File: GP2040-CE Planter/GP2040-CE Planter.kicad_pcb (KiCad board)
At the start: 4 copper layers, 50 x 50 mm, 57 parts, among them J1 USB_B, J2 USB_A, J3 USB_A, J4 USB_A, J5 USB_A, J6 USB_A, J7 Conn_01x02, U1 TUSB4041IPAPR, U3 TPS2561ADRCR, U4 TPS2561ADRCR, U5 PTMUXHS221NKGR

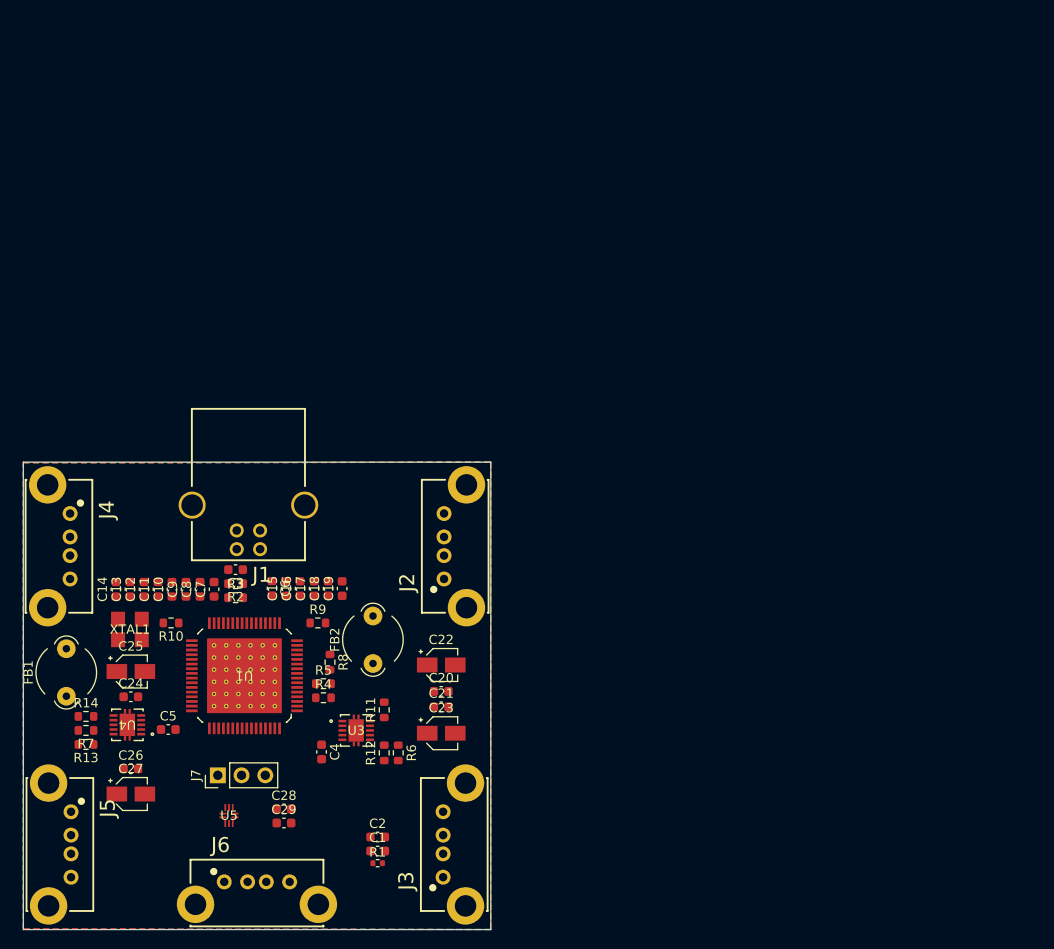
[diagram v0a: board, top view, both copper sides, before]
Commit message: Dueling Picos!
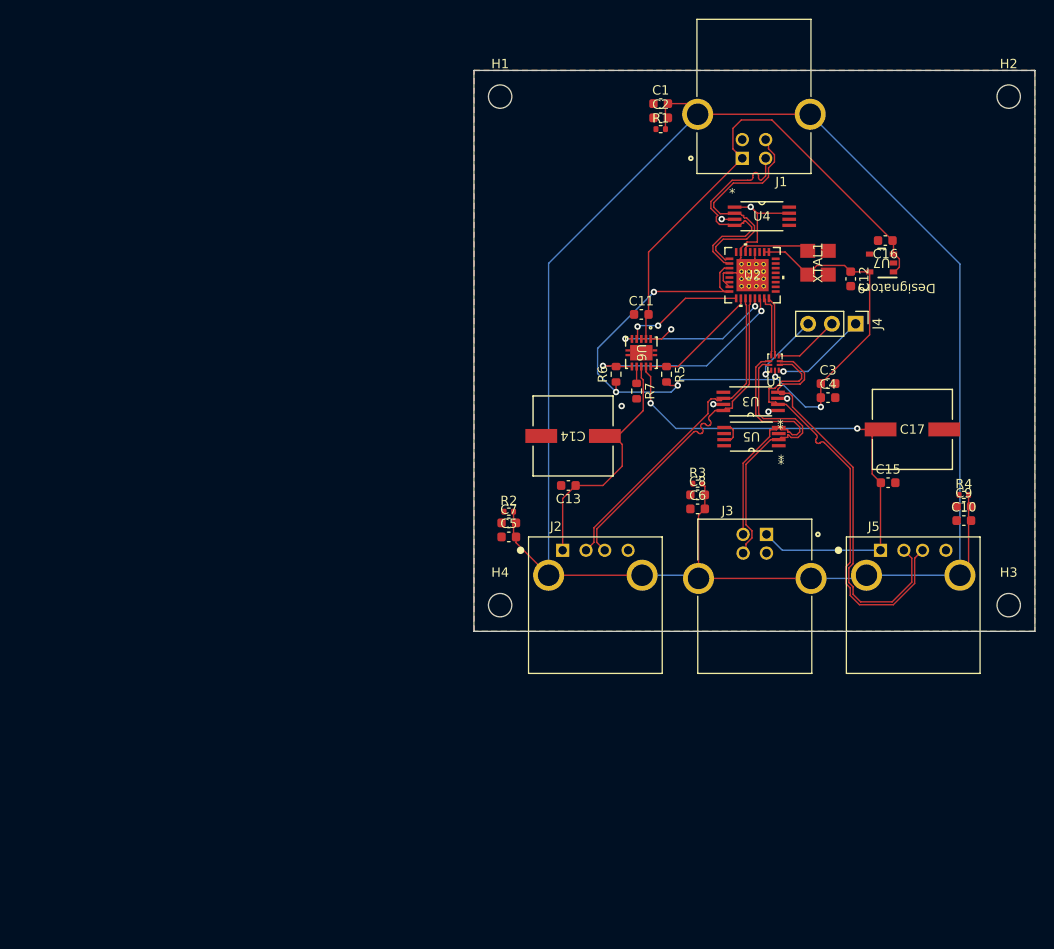
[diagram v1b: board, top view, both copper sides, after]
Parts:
- removed C18, C19: 01.μF, Capacitor_SMD:C_0603_1608Metric
- removed C20, C21, C24, C26, C29: 0.1μF, Capacitor_SMD:C_0603_1608Metric
- removed C22, C23, C25, C27: 150μF, Capacitor_SMD:CP_Elec_3x5.3
- removed C28: 1μF, Capacitor_SMD:C_0603_1608Metric
- removed FB1, FB2: 220 @ 100MHz, Ferrite_THT:LairdTech_28C0236-0JW-10
- removed J6: USB_A, GP2040-CE-Tester:GCT_USB1040-XX-X-X_REVC
- removed J7: Conn_01x02, Connector_PinHeader_2.54mm:PinHeader_1x03_P2.54mm_Vertical
- removed R10: 9.53K 1%, Resistor_SMD:R_0603_1608Metric
- removed R11, R12, R13, R14: 10K 5%, Resistor_SMD:R_0603_1608Metric
- removed R8, R9: 4.7K, Resistor_SMD:R_0603_1608Metric
- added H1: MountingHole, MountingHole:MountingHole_2.5mm, F.Cu at (110.8, 20.8)
- added H2: MountingHole, MountingHole:MountingHole_2.5mm, F.Cu at (165.2, 20.8)
- added H3: MountingHole, MountingHole:MountingHole_2.5mm, F.Cu at (165.2, 75.2)
- added H4: MountingHole, MountingHole:MountingHole_2.5mm, F.Cu at (110.8, 75.2)
- added U2: TUSB2046IBVF, GP2040-CE-Tester:RHB32_3P45X3P45_TEX, F.Cu at (137.8, 39.9)
- added U6: TPS2561ADRCR, GP2040-CE-Tester:DRC10_2P4X1P65_TEX, F.Cu at (125.9, 48.2)
- added U7: TLV73333PDBVR, GP2040-CE-Tester:TLV7333P, F.Cu at (151.6, 38.6)
- C1: value 0.1μF -> C
- C10, C11, C12, C13, C15, C16, C7, C8, C9: value 01.μF -> C
- C14, C17: value 01.μF -> C_Polarized_Small; footprint Capacitor_SMD:C_0603_1608Metric -> GP2040-CE-Tester:CAP_RHA&slash_HS_8X6P7_NCH
- C2: value 0.001μF -> C
- C3: value 10μF -> C
- C6: value 1μF -> C
- J1: value USB_B -> UJ2-BH-1-TH; footprint GP2040-CE-Tester:GCT_USB1030-XX-X-B-B_REVB -> GP2040-CE-Tester:CUI_UJ2-BH-1-TH
- J2, J5: value USB_A -> UJ2-AH-4-TH; footprint GP2040-CE-Tester:GCT_USB1040-XX-X-X_REVC -> GP2040-CE-Tester:CUI_UJ2-AH-4-TH
- J3: value USB_A -> UJ2-BH-1-TH; footprint GP2040-CE-Tester:GCT_USB1040-XX-X-X_REVC -> GP2040-CE-Tester:CUI_UJ2-BH-1-TH
- J4: value USB_A -> Conn_01x03; footprint GP2040-CE-Tester:GCT_USB1040-XX-X-X_REVC -> Connector_PinHeader_2.54mm:PinHeader_1x03_P2.54mm_Vertical
- R1: value 10KΩ 1% -> R
- R2: value 90.9KΩ 1% -> R; footprint Resistor_SMD:R_0603_1608Metric -> Resistor_SMD:R_0402_1005Metric
- R3: value 10KΩ 1% -> R; footprint Resistor_SMD:R_0603_1608Metric -> Resistor_SMD:R_0402_1005Metric
- R4: value 4.7K -> R; footprint Resistor_SMD:R_0603_1608Metric -> Resistor_SMD:R_0402_1005Metric
- R5: value 4.7K -> R
- R6, R7: value 25.5K 5% -> R
- U1: value TUSB4041IPAPR -> TMUXHS221NKGR; footprint GP2040-CE-Tester:TUSB4041I-Q1 -> GP2040-CE-Tester:TMUXHS221
- U3, U4: value TPS2561ADRCR -> SN75240PWR; footprint GP2040-CE-Tester:DRC10_2P4X1P65_TEX -> GP2040-CE-Tester:SN75240
- U5: value PTMUXHS221NKGR -> SN75240PWR; footprint GP2040-CE-Tester:TMUXHS221N -> GP2040-CE-Tester:SN75240
- XTAL1: value SIT1602AC-33-33E-24.000000Y -> SIT1602BC-33-33E-6.000000T; footprint GP2040-CE-Tester:SIT1602 -> GP2040-CE-Tester:SON4_SIT1602-3_SIT
- moved J5 94.4 mm to (151.5, 69.3), turned to 0 degrees
- moved J4 89.6 mm to (148.8, 45.1)
- moved U4 87.0 mm to (138.8, 33.6), turned to 0 degrees
- moved C1 85.5 mm to (128.0, 21.6)
- moved C10 85.0 mm to (160.4, 66.2), turned to 0 degrees
- moved R1 84.2 mm to (128.0, 24.3)
- moved C9 83.7 mm to (160.4, 64.6), turned to 0 degrees
- moved XTAL1 83.4 mm to (144.8, 38.6), turned to 90 degrees
- moved C2 82.7 mm to (128.0, 23.1)
- moved C12 82.6 mm to (148.3, 40.3), turned to -90 degrees
- moved C16 72.8 mm to (152.0, 36.2), turned to 180 degrees
- moved R4 71.9 mm to (160.4, 63.4)
- moved R7 69.2 mm to (125.4, 52.3), turned to -90 degrees
- moved U5 69.0 mm to (137.7, 57.2), turned to 180 degrees
- moved C3 66.4 mm to (145.9, 51.5), turned to 0 degrees
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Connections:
- C1 pad 1: Earth -> GND
- C1 pad 2: GND -> Earth
- C10 pad 1: Net-(C10-Pad1) -> GND
- C10 pad 2: GND -> Earth
- C11 pad 1: Net-(C10-Pad1) -> GND
- C11 pad 2: GND -> VBUS
- C12 pad 1: Net-(C10-Pad1) -> +3.3V
- C13 pad 1: Net-(C10-Pad1) -> /DN_1_VBUS
- C14 pad 1: Net-(C10-Pad1) -> /DN_1_VBUS
- C15 pad 1: Net-(C15-Pad1) -> /DN_2_VBUS
- C16 pad 1: Net-(C15-Pad1) -> VBUS
- C17 pad 1: Net-(C15-Pad1) -> /DN_2_VBUS
- C2 pad 1: Earth -> GND
- C2 pad 2: GND -> Earth
- C3 pad 1: VBUS -> +3.3V
- C4 pad 1: VBUS -> +3.3V
- C5 pad 1: VBUS -> GND
- C5 pad 2: GND -> Earth
- C6 pad 2: Net-(U1-GRST_N) -> Earth
- C7 pad 1: Net-(C10-Pad1) -> GND
- C7 pad 2: GND -> Earth
- C8 pad 1: Net-(C10-Pad1) -> GND
- C8 pad 2: GND -> Earth
- C9 pad 1: Net-(C10-Pad1) -> GND
- C9 pad 2: GND -> Earth
- J3 pad 2: /DN_2_D- -> /DB-
- J3 pad 3: /DN_2_D+ -> /DB+
- J4 pad 1: /DN_3_VBUS -> /SEL
- J4 pad 2: /DN_3_D- -> GND
- J4 pad 3: /DN_3_D+ -> /OEN
- J5 pad 1: /DN_4_VBUS -> /DN_2_VBUS
- J5 pad 2: /DN_4_D- -> /DN_2_D-
- J5 pad 3: /DN_4_D+ -> /DN_2_D+
- R1 pad 1: Earth -> GND
- R1 pad 2: GND -> Earth
- R2 pad 1: VBUS -> GND
- R2 pad 2: Net-(U1-USB_VBUS) -> Earth
- R3 pad 1: Net-(U1-USB_VBUS) -> GND
- R3 pad 2: GND -> Earth
- R4 pad 1: Net-(U1-FULLPWRMGMT_SMBA1_N) -> GND
- R4 pad 2: GND -> Earth
- R5 pad 1: Net-(U1-GANGED_SMBA2_HS_UP) -> /OVERCUR1_N
- R5 pad 2: GND -> +3.3V
- R6 pad 1: Net-(U3-ILIM) -> +3.3V
- R6 pad 2: GND -> /OVERCUR2_N
- R7 pad 1: Net-(U4-ILIM) -> Net-(U6-ILIM)
- U1 pad 1: /PWRCTL3_BATEN3 -> /DN_2_D+
- U1 pad 10: Net-(U1-GANGED_SMBA2_HS_UP) -> /SEL
- U1 pad 2: Net-(C15-Pad1) -> /DN_2_D-
- U1 pad 3: /PWRCTL2_BATEN2 -> GND
- U1 pad 4: /PWRCTL1_BATEN1 -> /DA+
- U1 pad 5: unconnected-(U1-SDA_SMBDAT-Pad5) -> /DA-
- U1 pad 6: unconnected-(U1-SCL_SMBCLK-Pad6) -> /DB-
- U1 pad 7: unconnected-(U1-SMBUS_N-Pad7) -> /DB+
- U1 pad 8: Net-(U1-FULLPWRMGMT_SMBA1_N) -> /OEN
- U1 pad 9: unconnected-(U1-PWRCTL_POL-Pad9) -> +3.3V
- U3 pad 2: VBUS -> /DN_2_D+
- U3 pad 3: VBUS -> GND
- U3 pad 4: /PWRCTL1_BATEN1 -> /DN_2_D-
- U3 pad 5: /PWRCTL2_BATEN2 -> GND
- U3 pad 6: /OVERCUR2_N -> /DN_1_D-
- U3 pad 7: Net-(U3-ILIM) -> GND
- U3 pad 8: /DN_2_VBUS -> /DN_1_D+
- U4 pad 2: VBUS -> /UP_D+
- U4 pad 3: VBUS -> GND
- U4 pad 4: /PWRCTL3_BATEN3 -> /UP_D-
- U4 pad 5: /PWRCTL4_BATEN4 -> GND
- U4 pad 6: /OVERCUR4_N -> unconnected-(U4-B-Pad6)
- U4 pad 7: Net-(U4-ILIM) -> GND
- U4 pad 8: /DN_4_VBUS -> unconnected-(U4-A-Pad8)
- U5 pad 1: /DN_2_D+ -> GND
- U5 pad 2: /DN_2_D- -> /DB+
- U5 pad 4: /DA+ -> /DB-
- U5 pad 5: /DA- -> GND
- U5 pad 6: /DB- -> unconnected-(U5-B-Pad6)
- U5 pad 7: /DB+ -> GND
- U5 pad 8: /OEN -> unconnected-(U5-A-Pad8)
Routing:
- net Earth: track 0.00 -> 202.5 mm
- net +3.3V: track 0.00 -> 83.1 mm, vias 0 -> 5
- net /DN_2_VBUS: track 0.00 -> 56.6 mm, vias 0 -> 2
- net VBUS: track 0.00 -> 54.6 mm
- net /DN_2_D+: track 0.00 -> 47.0 mm
- net /DN_2_D-: track 0.00 -> 44.8 mm
- net /DN_1_D+: track 0.00 -> 36.8 mm
- net /DN_1_D-: track 0.00 -> 35.5 mm
- net GND: track 0.00 -> 35.2 mm, vias 0 -> 7
- net /DB+: track 0.00 -> 30.2 mm
- net /DB-: track 0.00 -> 28.9 mm
- net /DN_1_VBUS: track 0.00 -> 27.9 mm
- net /UP_D+: track 0.00 -> 25.2 mm
- net /UP_D-: track 0.00 -> 25.1 mm
- net /OVERCUR2_N: track 0.00 -> 23.9 mm, vias 0 -> 2
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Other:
- board size 50 x 50 mm -> 60 x 60 mm
- rule pad_to_mask_clearance: 0 -> 0.0508
